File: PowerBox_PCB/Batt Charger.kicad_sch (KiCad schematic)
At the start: 20 parts, among them U10 BQ25887RGER

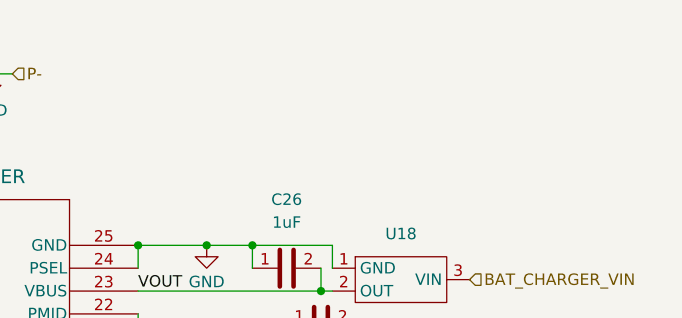
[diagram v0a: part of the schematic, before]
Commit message: Finished
Basically done
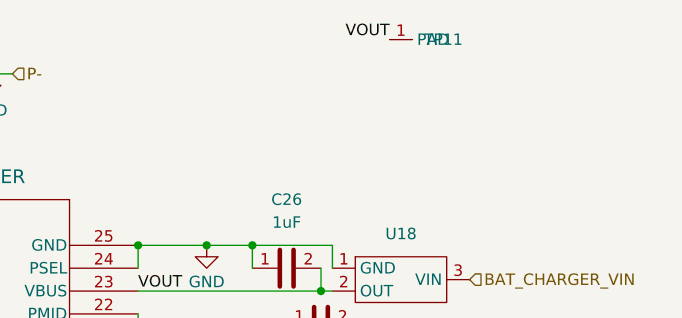
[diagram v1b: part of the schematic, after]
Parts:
- added TP11: (no value), Custom_Footprints:PAD-2x2, symbol Custom_Symbols:Pad-2x2
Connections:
- net VOUT: now also TP11.1 (PAD)
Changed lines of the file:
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@@
+		)
+	)
+	(label "VOUT"
+		(at 195.58 50.8 180)
+		(effects
+			(font
+				(size 1.27 1.27)
+			)
+			(justify right bottom)
 		)
 	)
@@
 					(unit 1)
 				)
+			)
+		)
+	)
+	(symbol
+		(lib_id "Custom_Symbols:Pad-2x2")
+		(at 198.12 50.8 90)
+		(unit 1)
+		(body_style 1)
+		(exclude_from_sim no)
+		(in_bom yes)
+		(on_board yes)
+		(in_pos_files yes)
+		(dnp no)
+		(fields_autoplaced yes)
+		(property "Reference" "TP11"
+			(at 199.39 50.7999 90)
+			(show_name no)
+			(do_not_autoplace no)
+			(effects
+				(font
+					(size 1.27 1.27)
+				)
+				(justify right)
+			)
+		)
+		(property "Value" ""
+			(at 198.12 50.8 0)
+			(show_name no)
+			(do_not_autoplace no)
+			(effects
+				(font
+					(size 1.27 1.27)
+				)
+			)
+		)
+		(property "Footprint" "Custom_Footprints:PAD-2x2"
+			(at 198.12 50.8 0)
+			(hide yes)
+			(show_name no)
+			(do_not_autoplace no)
+			(effects
+				(font
+					(size 1.27 1.27)
+				)
+			)
+		)
+		(property "Datasheet" ""
+			(at 198.12 50.8 0)
+			(hide yes)
+			(show_name no)
+			(do_not_autoplace no)
+			(effects
+				(font
+					(size 1.27 1.27)
+				)
+			)
+		)
+		(property "Description" ""
+			(at 198.12 50.8 0)
+			(hide yes)
+			(show_name no)
+			(do_not_autoplace no)
+			(effects
+				(font
+					(size 1.27 1.27)
+				)
+			)
+		)
+		(pin "1"
+		)
+		(instances
+			(project "PowerBox_PCB"
+				(path "/b0254e12-8cc0-427f-8cea-8f6ec8f66525/da3152ce-e99b-41cb-8d30-a5dc30414d8e"
+					(reference "TP11")
+					(unit 1)
+				)

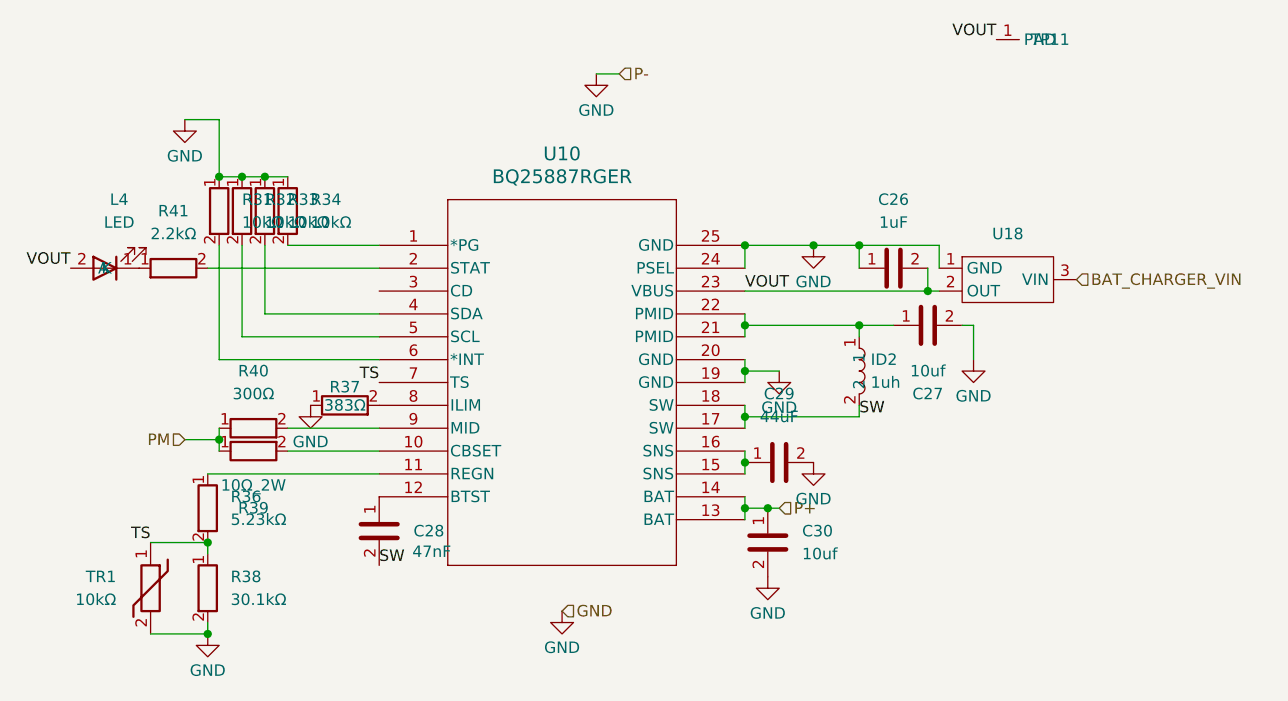
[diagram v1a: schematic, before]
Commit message: .
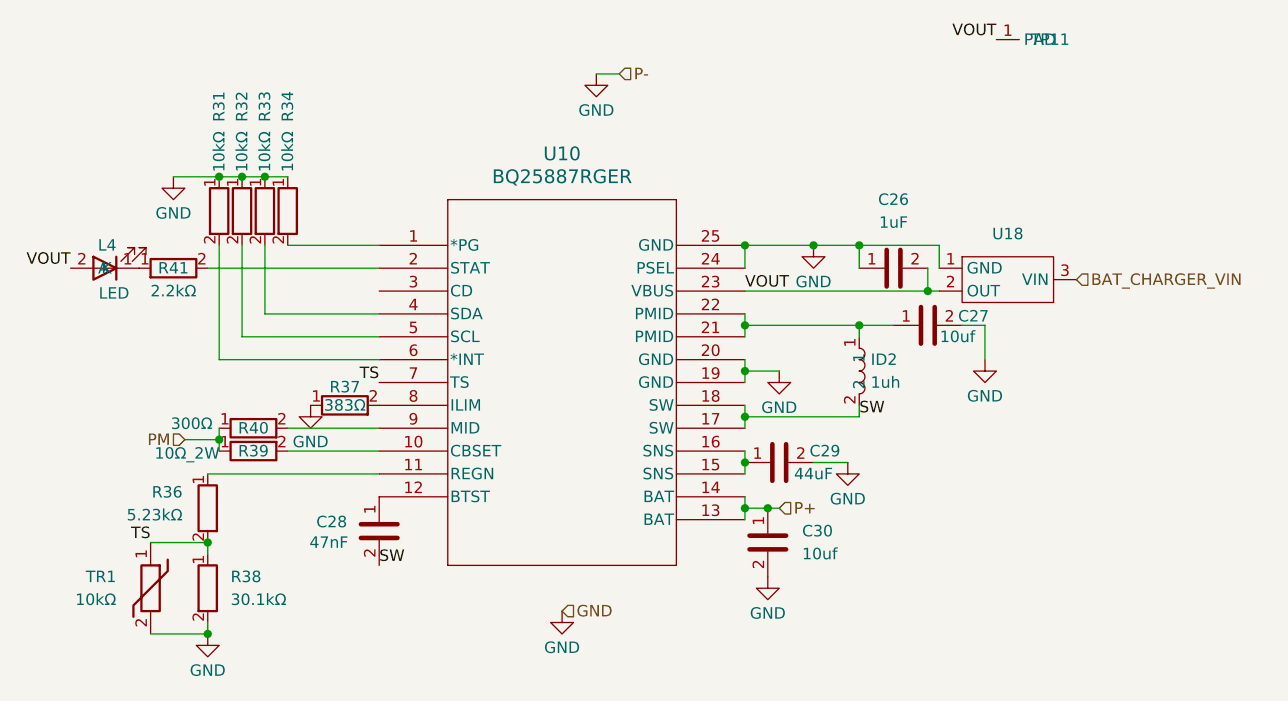
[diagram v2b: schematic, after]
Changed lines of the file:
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@@
+	(wire
+		(pts
+			(xy 179.07 97.79) (xy 175.26 97.79)
+		)
+		(stroke
+			(width 0)
+			(type default)
+		)
+	)
 	(wire
 		(pts
@@
 	(wire
 		(pts
-			(xy 109.22 66.04) (xy 109.22 59.69)
-		)
-		(stroke
-			(width 0)
-			(type default)
-		)
-	)
-	(wire
-		(pts
 			(xy 167.64 91.44) (xy 167.64 92.71)
 		)
@@
 	(wire
 		(pts
-			(xy 193.04 86.36) (xy 193.04 82.55)
+			(xy 194.31 86.36) (xy 194.31 82.55)
 		)
 		(stroke
@@
 	(wire
 		(pts
-			(xy 193.04 82.55) (xy 191.77 82.55)
+			(xy 194.31 82.55) (xy 191.77 82.55)
 		)
 		(stroke
@@
 	(wire
 		(pts
-			(xy 109.22 59.69) (xy 105.41 59.69)
+			(xy 109.22 66.04) (xy 104.14 66.04)
 		)
 		(stroke
@@
 	(symbol
 		(lib_id "power:GND")
-		(at 193.04 86.36 0)
+		(at 194.31 86.36 0)
 		(unit 1)
 		(body_style 1)
@@
 		(dnp no)
 		(property "Reference" "#PWR032"
-			(at 193.04 92.71 0)
+			(at 194.31 92.71 0)
 			(hide yes)
 			(show_name no)
@@
 		)
 		(property "Value" "GND"
-			(at 193.04 90.424 0)
+			(at 194.31 90.424 0)
 			(show_name no)
 			(do_not_autoplace no)
@@
 		)
 		(property "Footprint" ""
-			(at 193.04 86.36 0)
+			(at 194.31 86.36 0)
 			(hide yes)
 			(show_name no)
@@
 		)
 		(property "Datasheet" ""
-			(at 193.04 86.36 0)
+			(at 194.31 86.36 0)
 			(hide yes)
 			(show_name no)
@@
 		)
 		(property "Description" "Power symbol creates a global label with name \"GND\" , ground"
-			(at 193.04 86.36 0)
+			(at 194.31 86.36 0)
 			(hide yes)
 			(show_name no)
@@
 	(symbol
 		(lib_id "power:GND")
-		(at 105.41 59.69 0)
+		(at 104.14 66.04 0)
 		(unit 1)
 		(body_style 1)
@@
 		(dnp no)
 		(property "Reference" "#PWR042"
-			(at 105.41 66.04 0)
+			(at 104.14 72.39 0)
 			(hide yes)
 			(show_name no)
@@
 		)
 		(property "Value" "GND"
-			(at 105.41 63.754 0)
+			(at 104.14 70.104 0)
 			(show_name no)
 			(do_not_autoplace no)
@@
 		)
 		(property "Footprint" ""
-			(at 105.41 59.69 0)
+			(at 104.14 66.04 0)
 			(hide yes)
 			(show_name no)
@@
 		)
 		(property "Datasheet" ""
-			(at 105.41 59.69 0)
+			(at 104.14 66.04 0)
 			(hide yes)
 			(show_name no)
@@
 		)
 		(property "Description" "Power symbol creates a global label with name \"GND\" , ground"
-			(at 105.41 59.69 0)
+			(at 104.14 66.04 0)
 			(hide yes)
 			(show_name no)
@@
 		(in_pos_files yes)
 		(dnp no)
-		(fields_autoplaced yes)
 		(property "Reference" "C29"
-			(at 171.45 90.17 90)
+			(at 176.53 96.52 90)
 			(show_name no)
 			(do_not_autoplace no)
@@
 		)
 		(property "Value" "44uF"
-			(at 171.45 92.71 90)
+			(at 175.26 99.06 90)
 			(show_name no)
 			(do_not_autoplace no)
@@
 		(in_pos_files yes)
 		(dnp no)
-		(fields_autoplaced yes)
 		(property "Reference" "R33"
-			(at 116.84 68.5799 0)
+			(at 114.3 59.944 90)
 			(show_name no)
 			(do_not_autoplace no)
@@
 		)
 		(property "Value" "10kΩ"
-			(at 116.84 71.1199 0)
+			(at 114.3 65.532 90)
 			(show_name no)
 			(do_not_autoplace no)
@@
 		(in_pos_files yes)
 		(dnp no)
-		(fields_autoplaced yes)
 		(property "Reference" "R34"
-			(at 119.38 68.5799 0)
+			(at 116.84 59.944 90)
 			(show_name no)
 			(do_not_autoplace no)
@@
 		)
 		(property "Value" "10kΩ"
-			(at 119.38 71.1199 0)
+			(at 116.84 65.532 90)
 			(show_name no)
 			(do_not_autoplace no)
@@
 		(in_pos_files yes)
 		(dnp no)
-		(fields_autoplaced yes)
 		(property "Reference" "R31"
-			(at 111.76 68.5799 0)
+			(at 109.22 59.944 90)
 			(show_name no)
 			(do_not_autoplace no)
@@
 		)
 		(property "Value" "10kΩ"
-			(at 111.76 71.1199 0)
+			(at 109.22 65.532 90)
 			(show_name no)
 			(do_not_autoplace no)
@@
 		(dnp no)
 		(property "Reference" "R39"
-			(at 113.03 102.87 90)
+			(at 113.03 96.52 90)
 			(show_name no)
 			(do_not_autoplace no)
@@
 		)
 		(property "Value" "10Ω_2W"
-			(at 113.03 100.33 90)
+			(at 105.664 96.774 90)
 			(show_name no)
 			(do_not_autoplace no)
@@
 		(lib_id "Custom_Symbols:5.23kRes")
 		(at 107.95 102.87 0)
-		(unit 1)
-		(body_style 1)
-		(exclude_from_sim no)
-		(in_bom yes)
-		(on_board yes)
-		(in_pos_files yes)
-		(dnp no)
-		(fields_autoplaced yes)
+		(mirror y)
+		(unit 1)
+		(body_style 1)
+		(exclude_from_sim no)
+		(in_bom yes)
+		(on_board yes)
+		(in_pos_files yes)
+		(dnp no)
 		(property "Reference" "R36"
-			(at 110.49 101.5999 0)
+			(at 105.156 101.092 0)
 			(show_name no)
 			(do_not_autoplace no)
@@
 		)
 		(property "Value" "5.23kΩ"
-			(at 110.49 104.1399 0)
+			(at 105.156 103.632 0)
 			(show_name no)
 			(do_not_autoplace no)
@@
 		(in_pos_files yes)
 		(dnp no)
-		(fields_autoplaced yes)
 		(property "Reference" "R32"
-			(at 114.3 68.5799 0)
+			(at 111.76 59.944 90)
 			(show_name no)
 			(do_not_autoplace no)
@@
 		)
 		(property "Value" "10kΩ"
-			(at 114.3 71.1199 0)
+			(at 111.76 65.532 90)
 			(show_name no)
 			(do_not_autoplace no)
@@
 		(dnp no)
 		(property "Reference" "C27"
-			(at 187.96 90.17 90)
+			(at 193.04 81.534 90)
 			(show_name no)
 			(do_not_autoplace no)
@@
 		)
 		(property "Value" "10uf"
-			(at 187.96 87.63 90)
+			(at 191.262 83.82 90)
 			(show_name no)
 			(do_not_autoplace no)
@@
 	(symbol
 		(lib_id "power:GND")
-		(at 175.26 97.79 0)
+		(at 179.07 97.79 0)
 		(unit 1)
 		(body_style 1)
@@
 		(dnp no)
 		(property "Reference" "#PWR037"
-			(at 175.26 104.14 0)
+			(at 179.07 104.14 0)
 			(hide yes)
 			(show_name no)
@@
 		)
 		(property "Value" "GND"
-			(at 175.26 101.854 0)
+			(at 179.07 101.854 0)
 			(show_name no)
 			(do_not_autoplace no)
@@
 		)
 		(property "Footprint" ""
-			(at 175.26 97.79 0)
+			(at 179.07 97.79 0)
 			(hide yes)
 			(show_name no)
@@
 		)
 		(property "Datasheet" ""
-			(at 175.26 97.79 0)
+			(at 179.07 97.79 0)
 			(hide yes)
 			(show_name no)
@@
 		)
 		(property "Description" "Power symbol creates a global label with name \"GND\" , ground"
-			(at 175.26 97.79 0)
+			(at 179.07 97.79 0)
 			(hide yes)
 			(show_name no)
@@
 		(in_pos_files yes)
 		(dnp no)
-		(fields_autoplaced yes)
 		(property "Reference" "R40"
-			(at 113.03 87.63 90)
+			(at 113.03 93.98 90)
 			(show_name no)
 			(do_not_autoplace no)
@@
 		)
 		(property "Value" "300Ω"
-			(at 113.03 90.17 90)
+			(at 106.172 93.472 90)
 			(show_name no)
 			(do_not_autoplace no)
@@
 		(lib_id "Custom_Symbols:47nF_Cap")
 		(at 127 105.41 0)
+		(mirror y)
 		(unit 1)
 		(body_style 1)
@@
 		(dnp no)
 		(property "Reference" "C28"
-			(at 130.81 105.4099 0)
+			(at 123.444 104.394 0)
 			(show_name no)
 			(do_not_autoplace no)
@@
 		)
 		(property "Value" "47nF"
-			(at 132.842 107.696 0)
+			(at 121.412 106.6801 0)
 			(show_name no)
 			(do_not_autoplace no)
@@
 		)
 		(property "Footprint" "Capacitor_SMD:C_0805_2012Metric_Pad1.18x1.45mm_HandSolder"
-			(at 127.254 105.41 0)
+			(at 126.746 105.41 0)
 			(hide yes)
 			(show_name no)
@@
 		(in_pos_files yes)
 		(dnp no)
-		(fields_autoplaced yes)
 		(property "Reference" "R41"
-			(at 104.14 69.85 90)
+			(at 104.14 76.2 90)
 			(show_name no)
 			(do_not_autoplace no)
@@
 		)
 		(property "Value" "2.2kΩ"
-			(at 104.14 72.39 90)
+			(at 104.14 78.74 90)
 			(show_name no)
 			(do_not_autoplace no)
@@
 		(in_pos_files yes)
 		(dnp no)
-		(fields_autoplaced yes)
 		(property "Reference" "L4"
-			(at 98.1075 68.58 0)
+			(at 96.774 73.66 0)
 			(show_name no)
 			(do_not_autoplace no)
@@
 		)
 		(property "Value" "LED"
-			(at 98.1075 71.12 0)
-			(show_name no)
-			(do_not_autoplace no)
+			(at 97.536 78.994 0)
+			(show_name no)
+			(do_not_autoplace no)
